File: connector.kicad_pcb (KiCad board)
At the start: 2 copper layers, 26.8 x 9.7 mm, 3 parts, among them J1 Conn_01x02, SW1 SW_Push

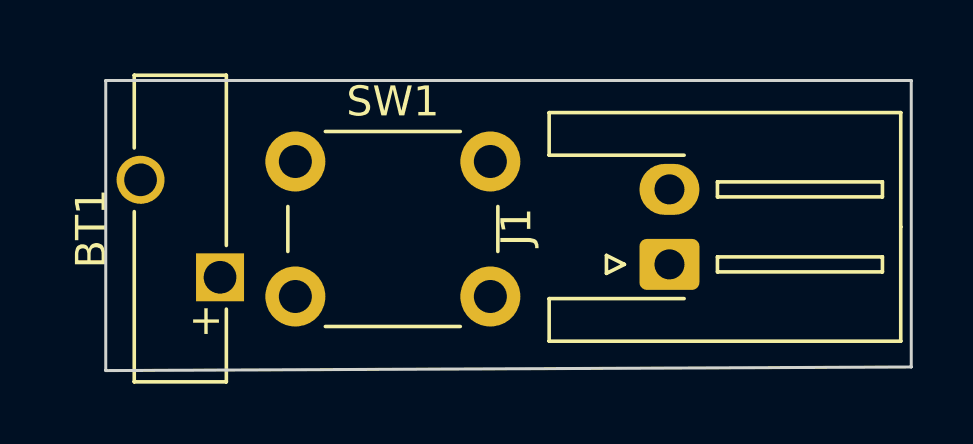
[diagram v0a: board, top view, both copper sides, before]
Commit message: feat: update the jst package
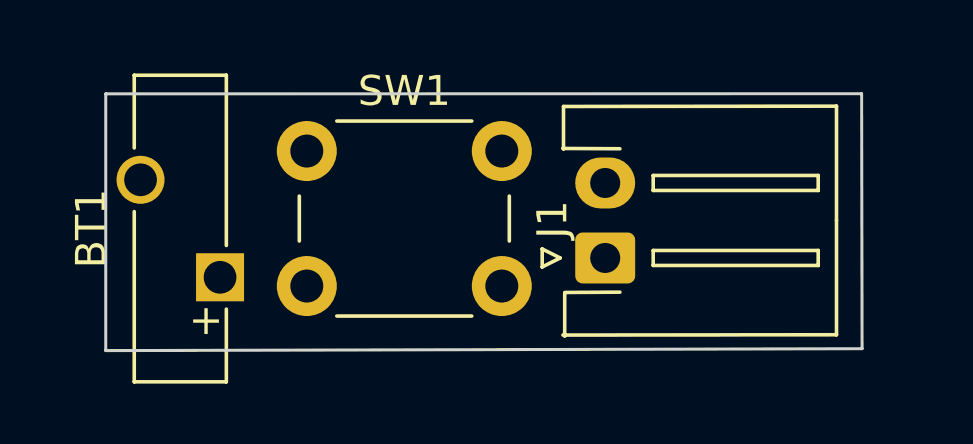
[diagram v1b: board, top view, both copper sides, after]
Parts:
- J1: footprint Connector_JST:JST_XH_S2B-XH-A-1_1x02_P2.50mm_Horizontal -> keyboard:JST_XH_S2B-XH-A-1_1x02_P2.50mm_Horizontal
- moved J1 2.15 mm to (165.8, 91.5)
- moved SW1 0.52 mm to (155.9, 87.9)
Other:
- board size 26.8 x 9.7 mm -> 25.2 x 8.6 mm
